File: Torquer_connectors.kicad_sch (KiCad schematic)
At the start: 3 parts

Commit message: I2C lines are pulled up
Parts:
- JT1, JT2, JT3: footprint (none) -> 502352-0210:5023520210
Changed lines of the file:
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@@
     (property "Reference" "JT2" (id 0) (at 50.8 43.18 0))
     (property "Value" "502352-0210" (id 1) (at 50.8 45.72 0))
-    (property "Footprint" "" (id 2) (at 39.37 55.88 0)
+    (property "Footprint" "502352-0210:5023520210" (id 2) (at 39.37 55.88 0)
       (effects (font (size 1.27 1.27)) hide)
     )
@@
     (property "Reference" "JT1" (id 0) (at 50.8 19.05 0))
     (property "Value" "502352-0210" (id 1) (at 50.8 21.59 0))
-    (property "Footprint" "" (id 2) (at 39.37 31.75 0)
+    (property "Footprint" "502352-0210:5023520210" (id 2) (at 39.37 31.75 0)
       (effects (font (size 1.27 1.27)) hide)
     )
@@
   (symbol (lib_id "upsat-comms-hardware:GND") (at 36.83 62.23 0) (unit 1)
     (in_bom yes) (on_board yes) (fields_autoplaced)
-    (property "Reference" "#PWR0159" (id 0) (at 36.83 68.58 0)
+    (property "Reference" "#PWR0160" (id 0) (at 36.83 68.58 0)
       (effects (font (size 1.27 1.27)) hide)
     )
@@
     (property "Reference" "JT3" (id 0) (at 52.07 69.85 0))
     (property "Value" "502352-0210" (id 1) (at 52.07 72.39 0))
-    (property "Footprint" "" (id 2) (at 40.64 82.55 0)
+    (property "Footprint" "502352-0210:5023520210" (id 2) (at 40.64 82.55 0)
       (effects (font (size 1.27 1.27)) hide)
     )
@@
   (symbol (lib_id "upsat-comms-hardware:GND") (at 35.56 35.56 0) (unit 1)
     (in_bom yes) (on_board yes) (fields_autoplaced)
-    (property "Reference" "#PWR0158" (id 0) (at 35.56 41.91 0)
+    (property "Reference" "#PWR0159" (id 0) (at 35.56 41.91 0)
       (effects (font (size 1.27 1.27)) hide)
     )
@@
   (symbol (lib_id "upsat-comms-hardware:GND") (at 39.37 87.63 0) (unit 1)
     (in_bom yes) (on_board yes) (fields_autoplaced)
-    (property "Reference" "#PWR0160" (id 0) (at 39.37 93.98 0)
+    (property "Reference" "#PWR0161" (id 0) (at 39.37 93.98 0)
       (effects (font (size 1.27 1.27)) hide)
     )

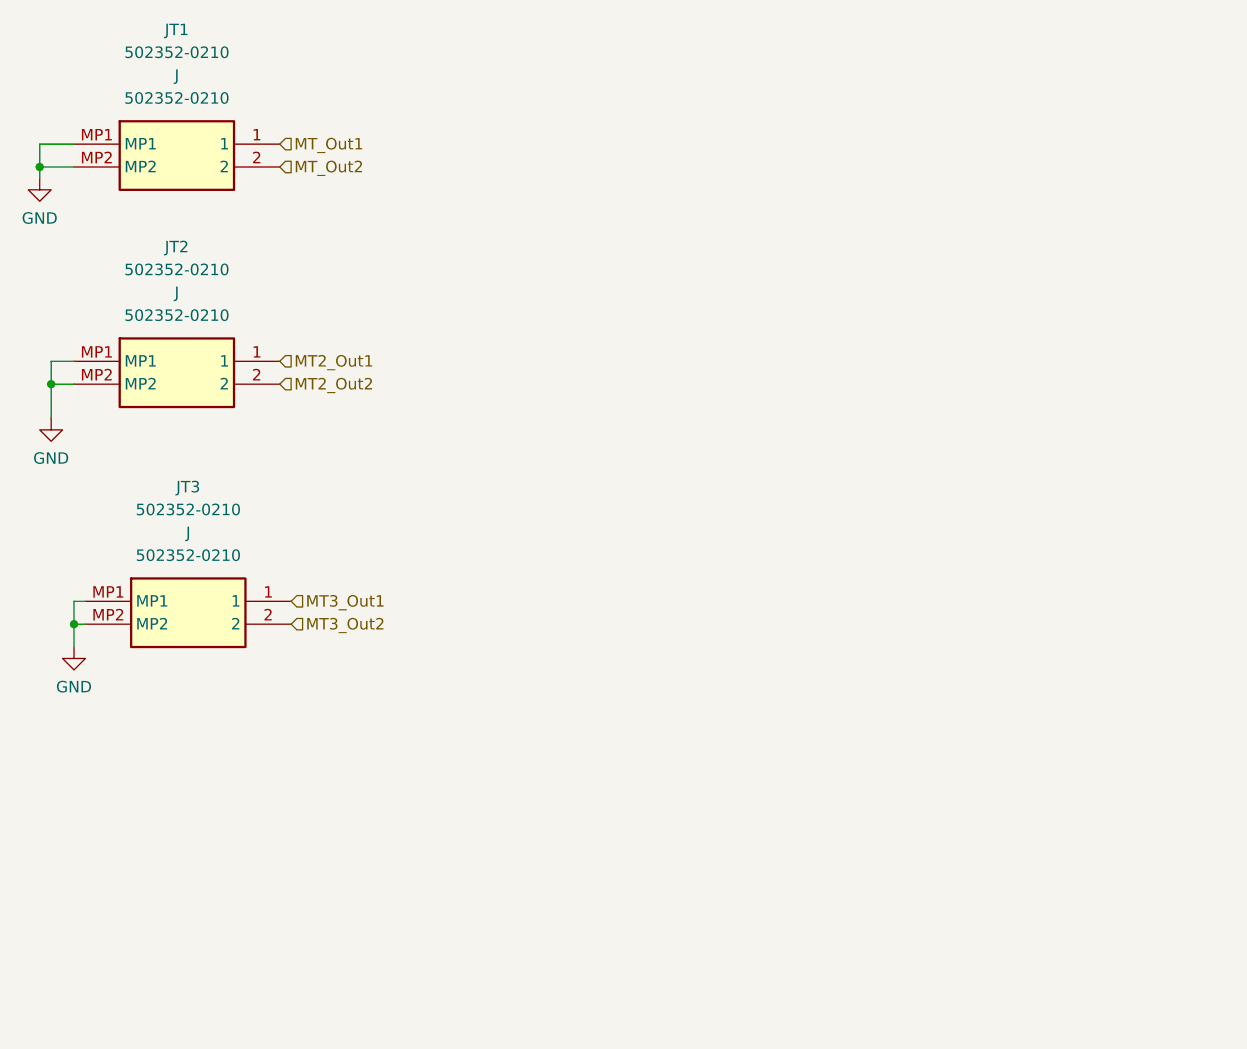
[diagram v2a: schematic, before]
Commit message: Final Schematic
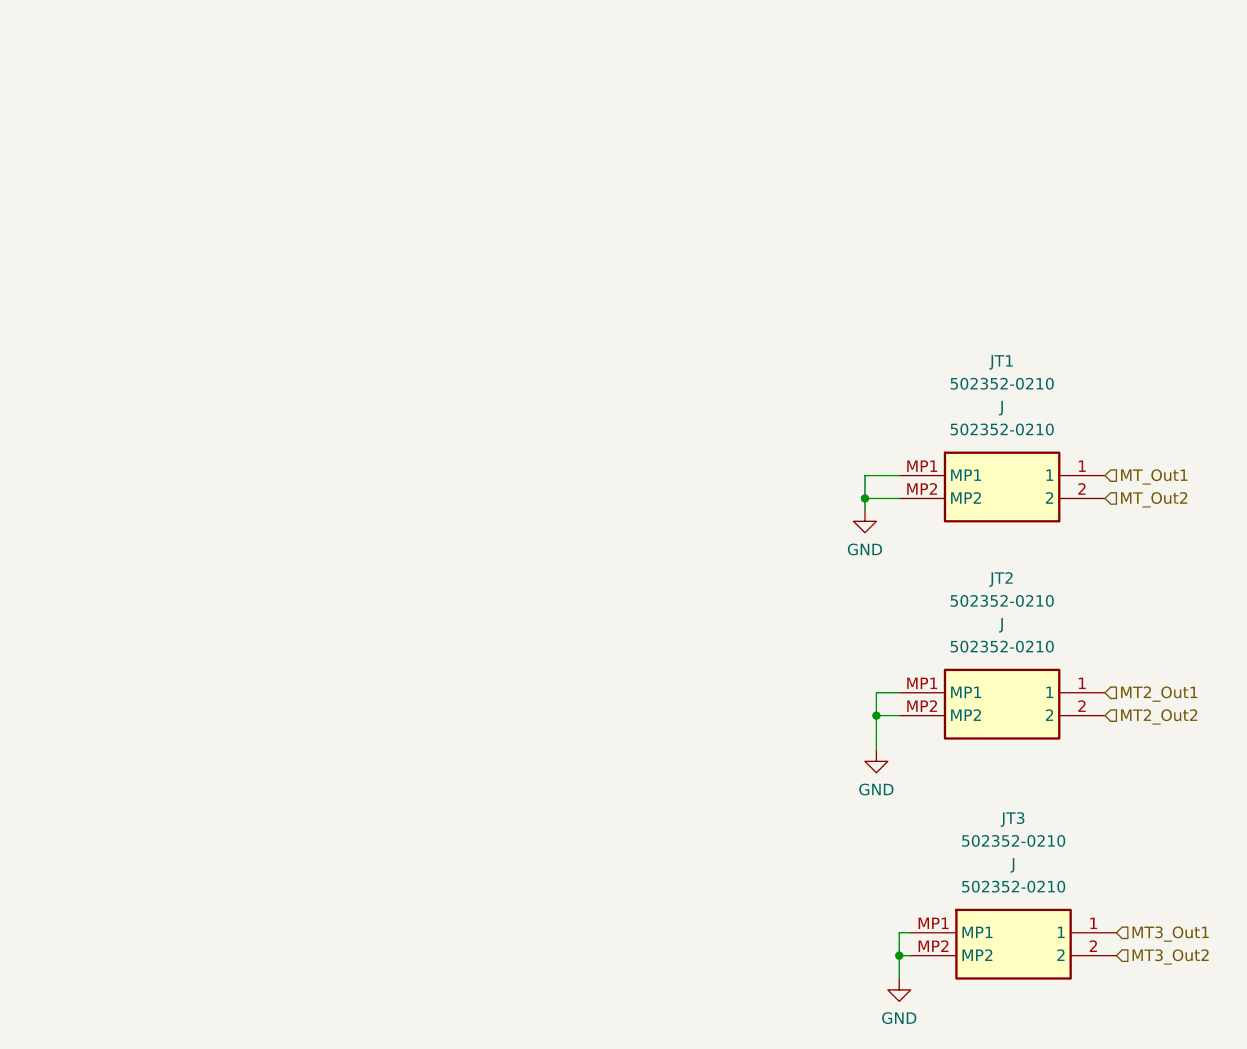
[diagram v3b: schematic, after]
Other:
- moved on the sheet: JT1, JT2, JT3
